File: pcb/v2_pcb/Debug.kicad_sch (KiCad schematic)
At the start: 5 parts, among them J1 Conn_ARM_SWD_TagConnect_TC203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, SW301 DEV BOOT

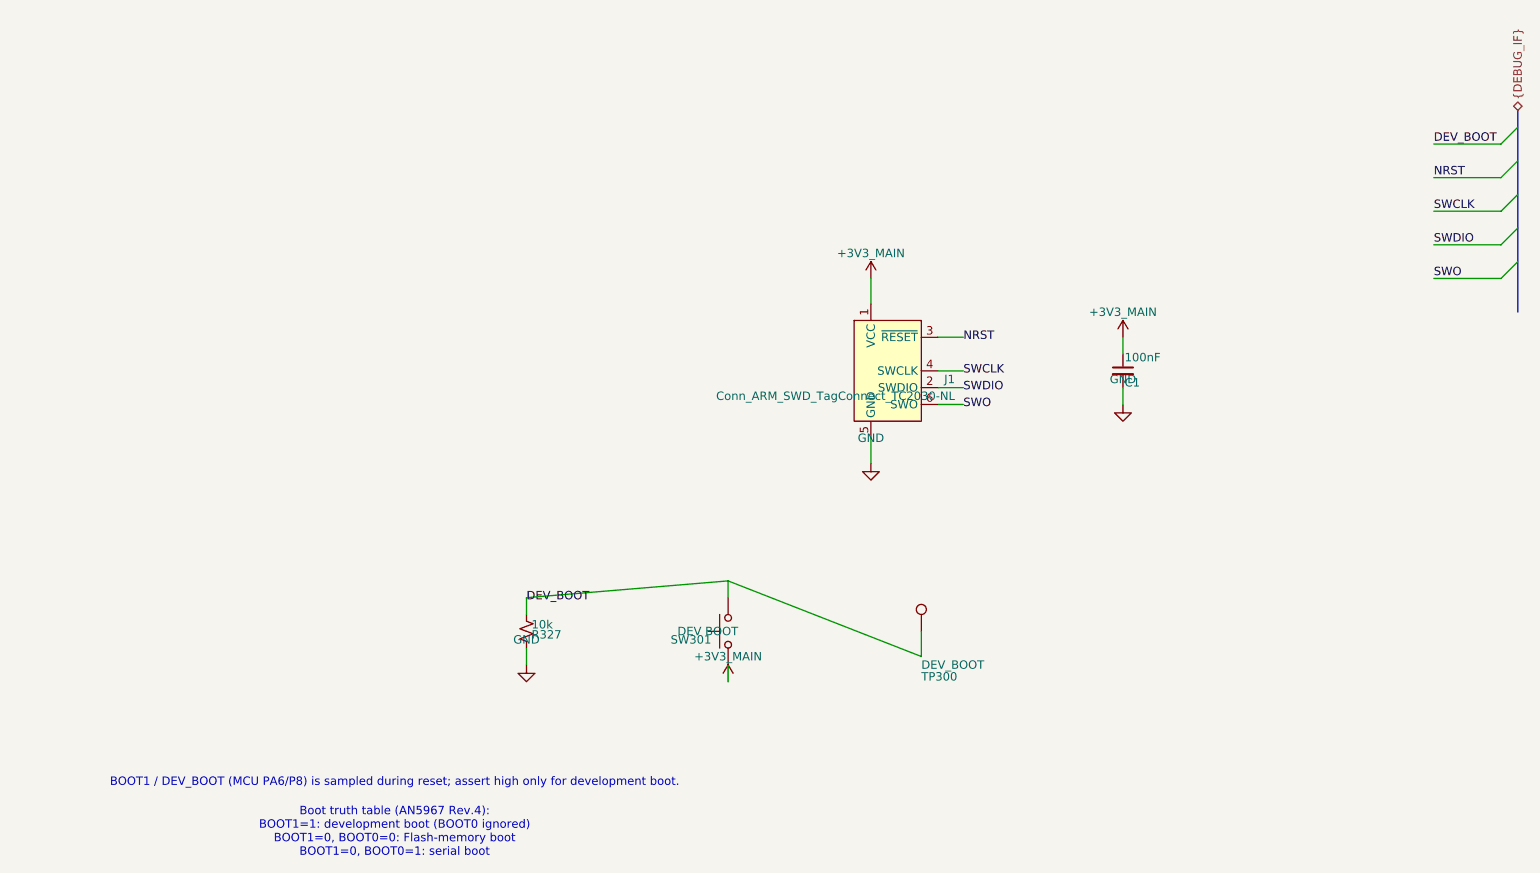
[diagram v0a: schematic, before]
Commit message: power and debug cleanup
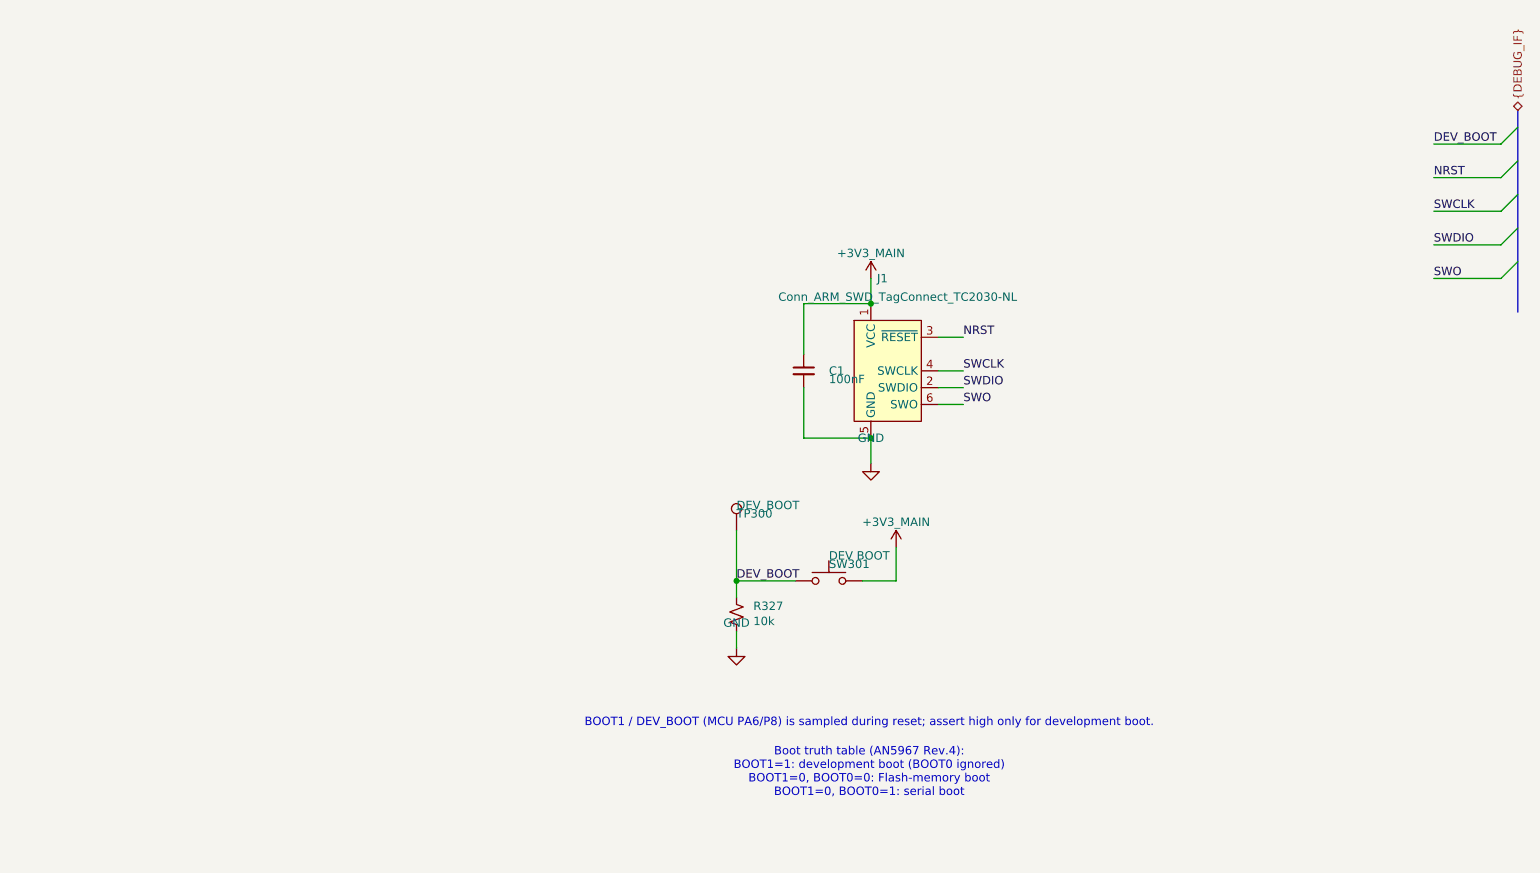
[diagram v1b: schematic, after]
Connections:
- net +3V3_MAIN: now also SW301.2; no longer SW301.1
- net DEV_BOOT: now also SW301.1; no longer SW301.2
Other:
- moved on the sheet: C1, R327, SW301, TP300
